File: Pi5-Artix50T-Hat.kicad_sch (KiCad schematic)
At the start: 0 parts

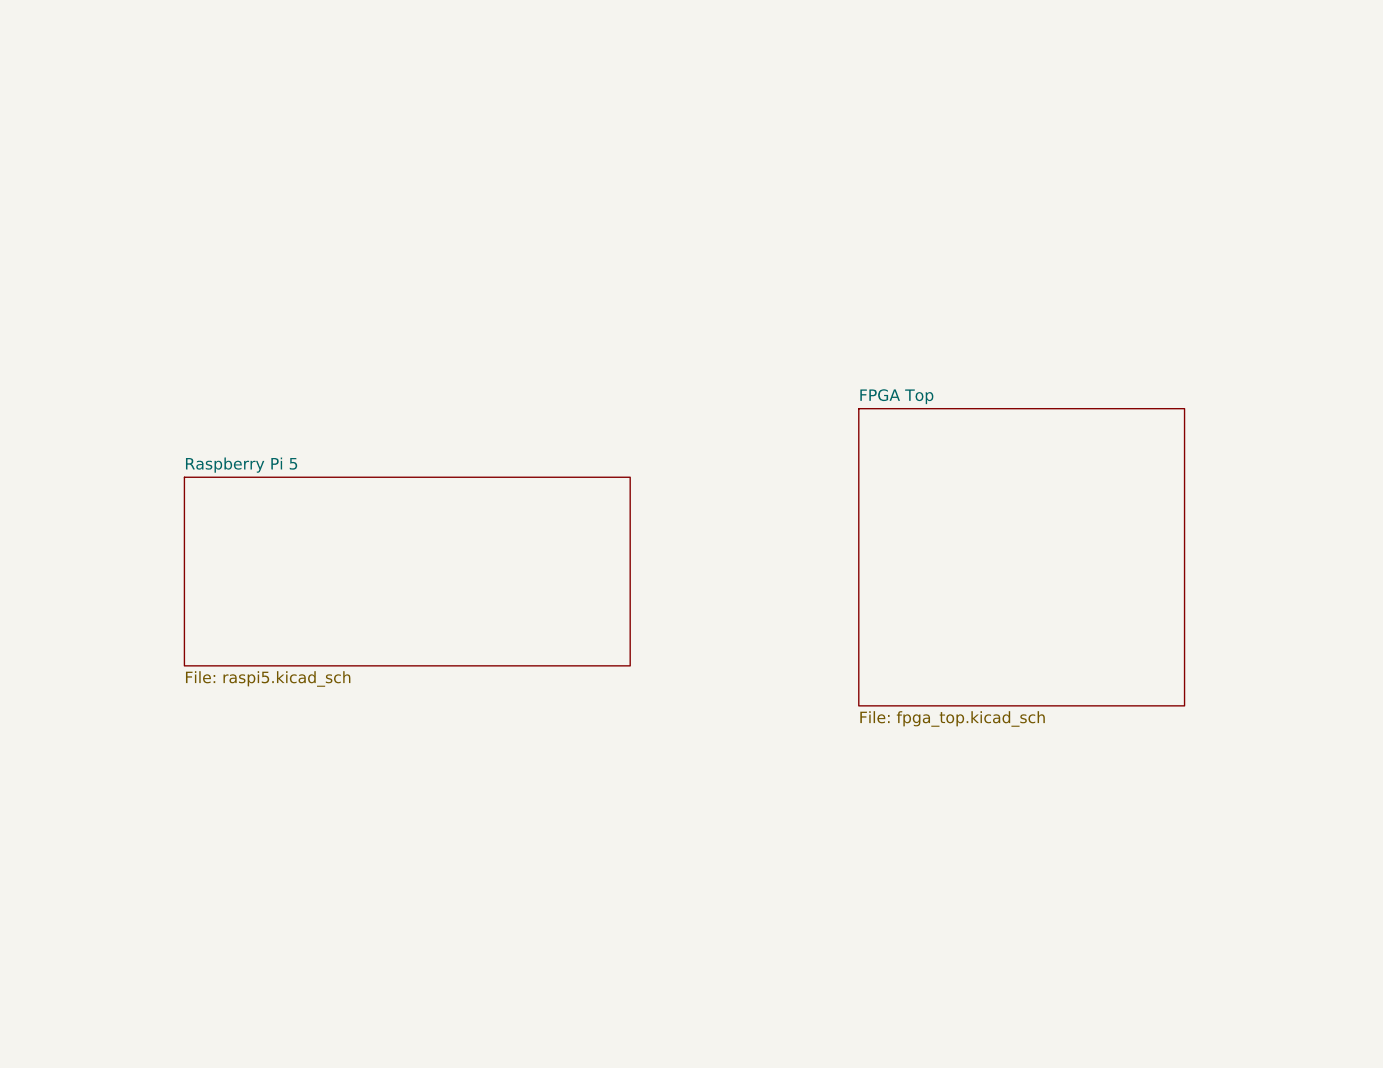
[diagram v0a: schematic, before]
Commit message: Schematic finished, starting layout
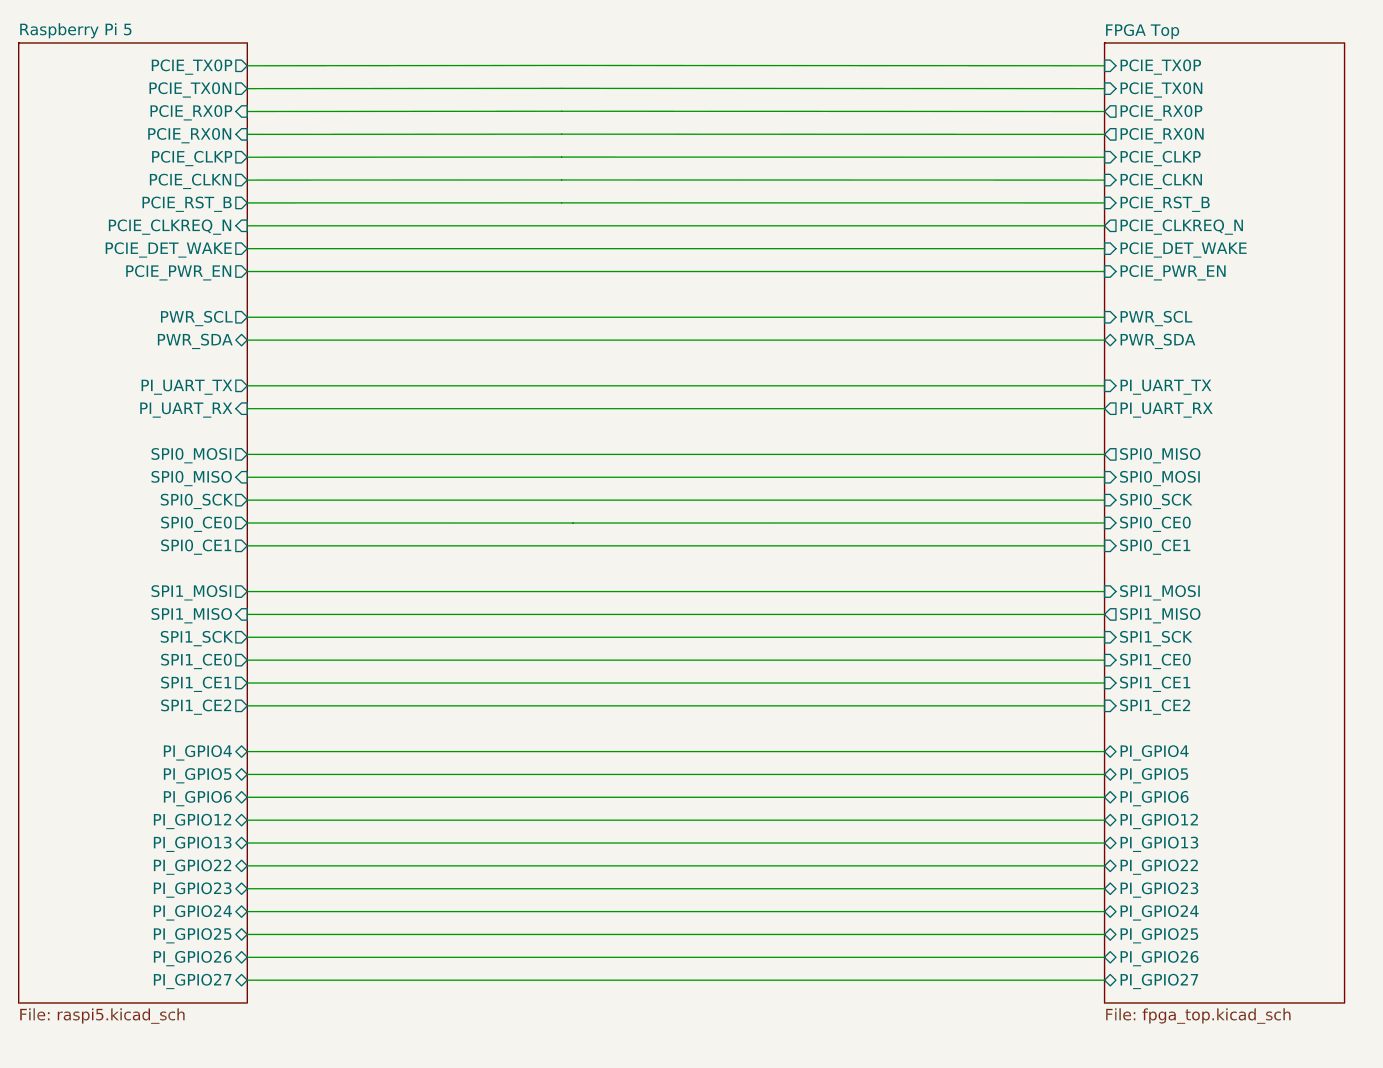
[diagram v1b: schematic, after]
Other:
- sheet FPGA Top ports: added PCIE_CLKN, PCIE_CLKP, PCIE_CLKREQ_N, PCIE_DET_WAKE, PCIE_PWR_EN, PCIE_RST_B, PCIE_RX0N, PCIE_RX0P, PCIE_TX0N, PCIE_TX0P, PI_GPIO12, PI_GPIO13, PI_GPIO22, PI_GPIO23, PI_GPIO24, PI_GPIO25, PI_GPIO26, PI_GPIO27, PI_GPIO4, PI_GPIO5, PI_GPIO6, PI_UART_RX, PI_UART_TX, PWR_SCL, PWR_SDA, SPI0_CE0, SPI0_CE1, SPI0_MISO, SPI0_MOSI, SPI0_SCK, SPI1_CE0, SPI1_CE1, SPI1_CE2, SPI1_MISO, SPI1_MOSI, SPI1_SCK; removed none
- sheet Raspberry Pi 5 ports: added PCIE_CLKN, PCIE_CLKP, PCIE_CLKREQ_N, PCIE_DET_WAKE, PCIE_PWR_EN, PCIE_RST_B, PCIE_RX0N, PCIE_RX0P, PCIE_TX0N, PCIE_TX0P, PI_GPIO12, PI_GPIO13, PI_GPIO22, PI_GPIO23, PI_GPIO24, PI_GPIO25, PI_GPIO26, PI_GPIO27, PI_GPIO4, PI_GPIO5, PI_GPIO6, PI_UART_RX, PI_UART_TX, PWR_SCL, PWR_SDA, SPI0_CE0, SPI0_CE1, SPI0_MISO, SPI0_MOSI, SPI0_SCK, SPI1_CE0, SPI1_CE1, SPI1_CE2, SPI1_MISO, SPI1_MOSI, SPI1_SCK; removed none
- title: Raspberry Pi 5 Artix 50T FPGA Hat - Top Level -> FPGA Power

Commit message: Updated titleblock texts
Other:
- title: FPGA Power -> Pi 5 - Artix XC7A50T - PCIe FPGA Hat
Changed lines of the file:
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@@
   (paper "A4")
   (title_block
-    (title "FPGA Power")
-    (date "2024-02-11")
+    (title "Pi 5 - Artix XC7A50T - PCIe FPGA Hat")
+    (date "2024-02-14")
     (rev "0.1")
     (company "George Smart, M1GEO")

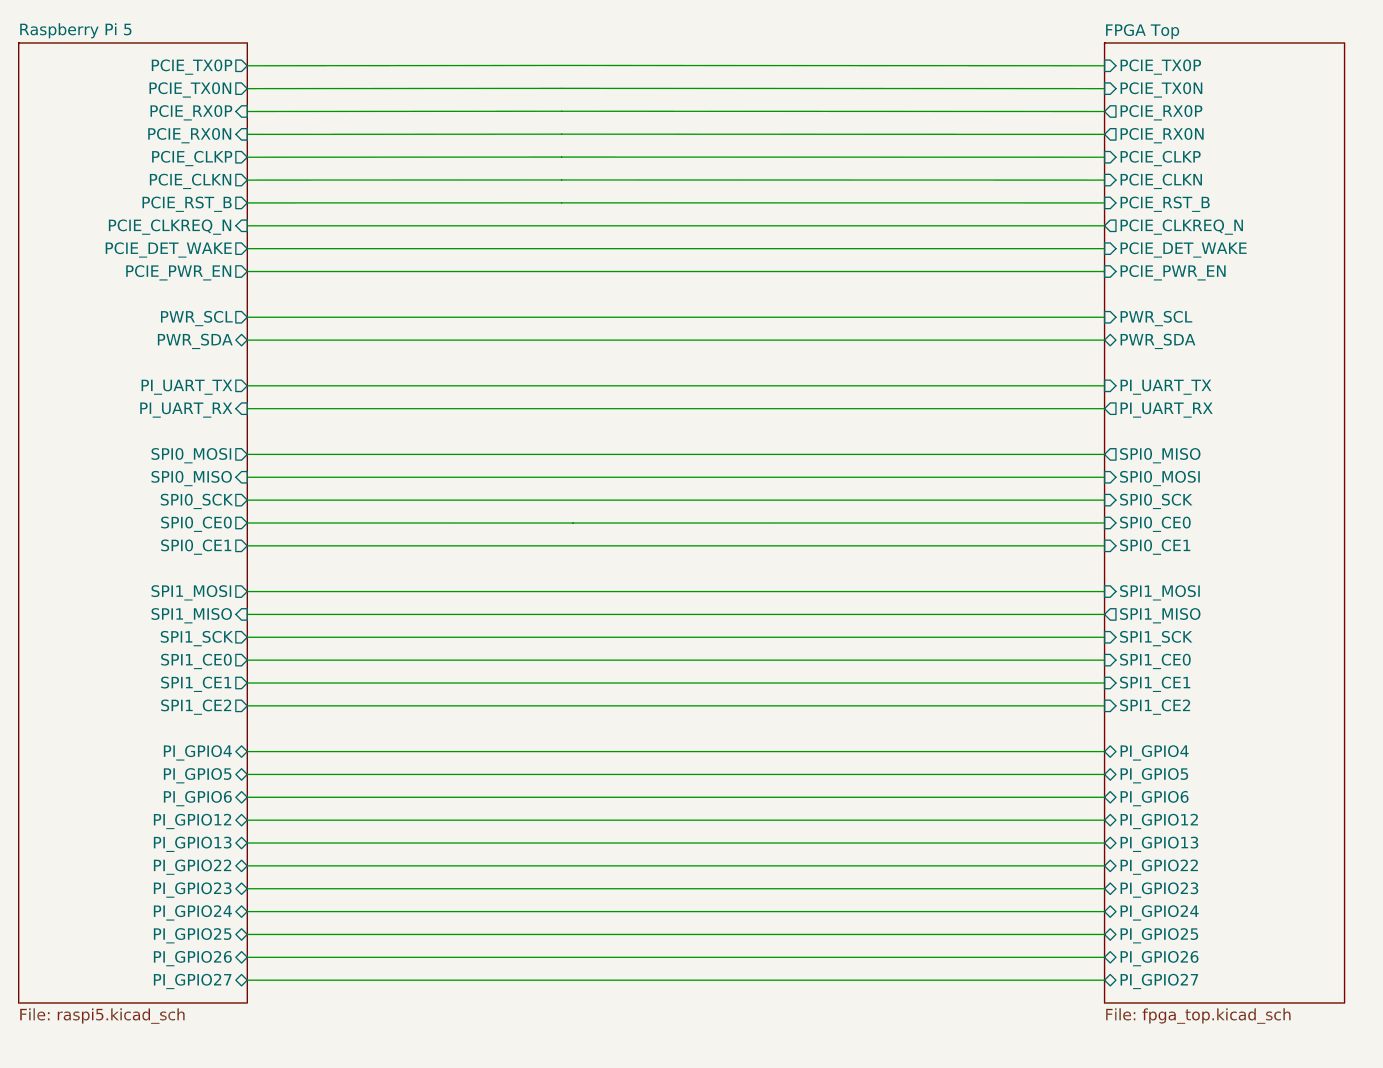
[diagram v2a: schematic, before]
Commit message: Started routing. More to go
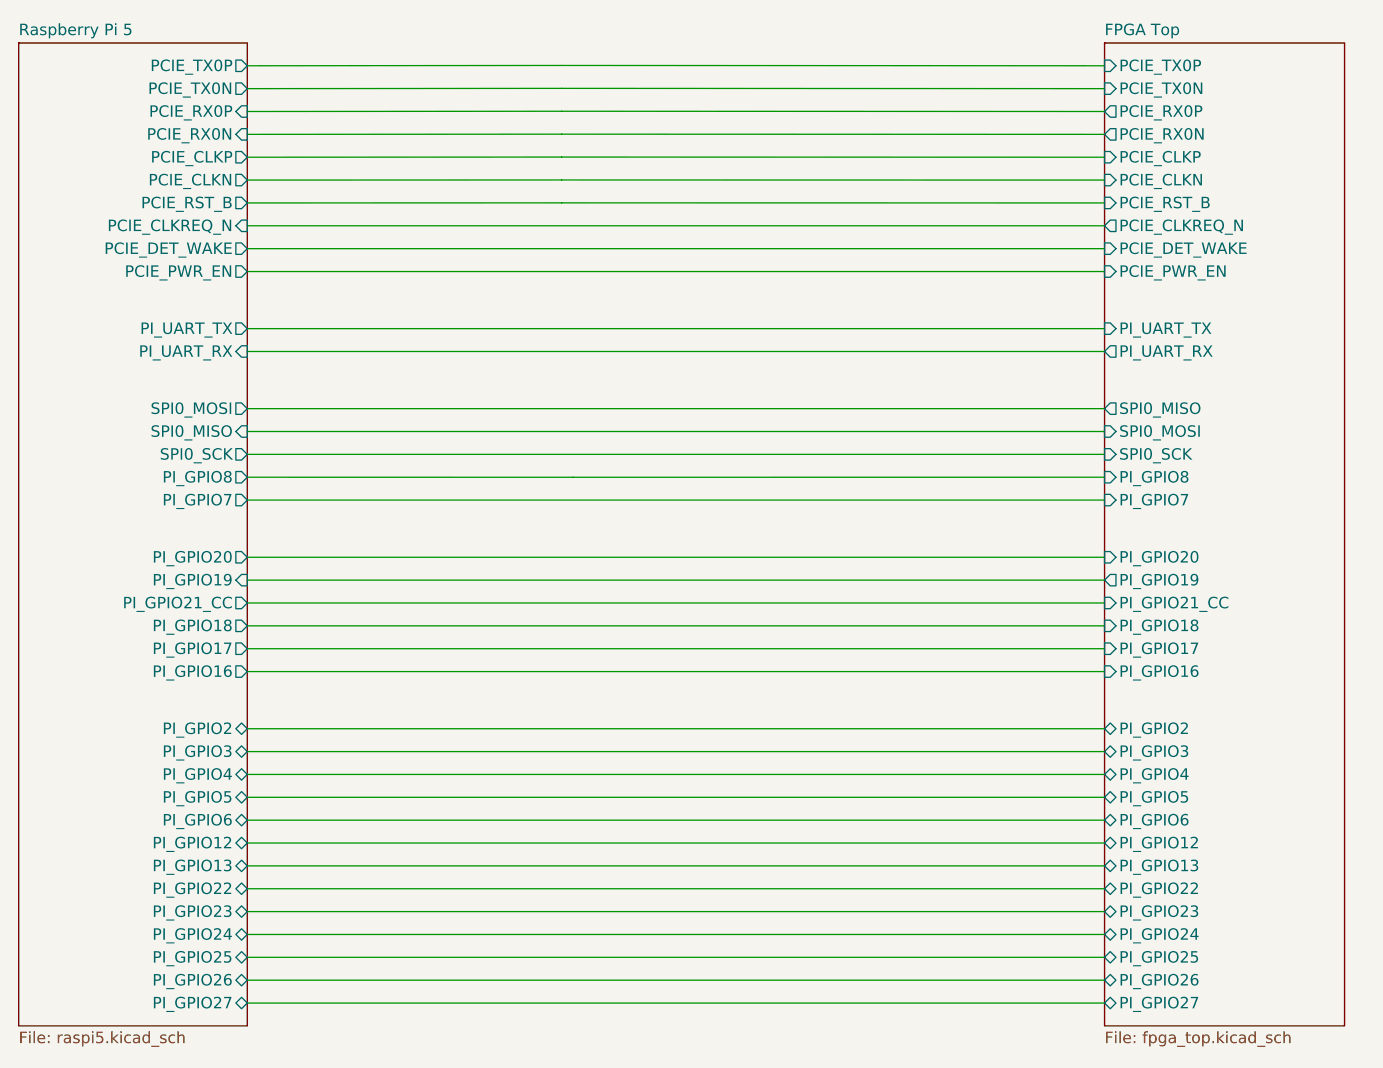
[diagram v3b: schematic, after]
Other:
- sheet FPGA Top ports: added PI_GPIO16, PI_GPIO17, PI_GPIO18, PI_GPIO19, PI_GPIO2, PI_GPIO20, PI_GPIO21_CC, PI_GPIO3, PI_GPIO7, PI_GPIO8; removed PWR_SCL, PWR_SDA, SPI0_CE0, SPI0_CE1, SPI1_CE0, SPI1_CE1, SPI1_CE2, SPI1_MISO, SPI1_MOSI, SPI1_SCK
- sheet Raspberry Pi 5 ports: added PI_GPIO16, PI_GPIO17, PI_GPIO18, PI_GPIO19, PI_GPIO2, PI_GPIO20, PI_GPIO21_CC, PI_GPIO3, PI_GPIO7, PI_GPIO8; removed PWR_SCL, PWR_SDA, SPI0_CE0, SPI0_CE1, SPI1_CE0, SPI1_CE1, SPI1_CE2, SPI1_MISO, SPI1_MOSI, SPI1_SCK
